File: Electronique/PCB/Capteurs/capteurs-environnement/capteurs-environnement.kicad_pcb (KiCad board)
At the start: 2 copper layers, 99.1 x 66 mm, 22 parts, among them U1 Pico

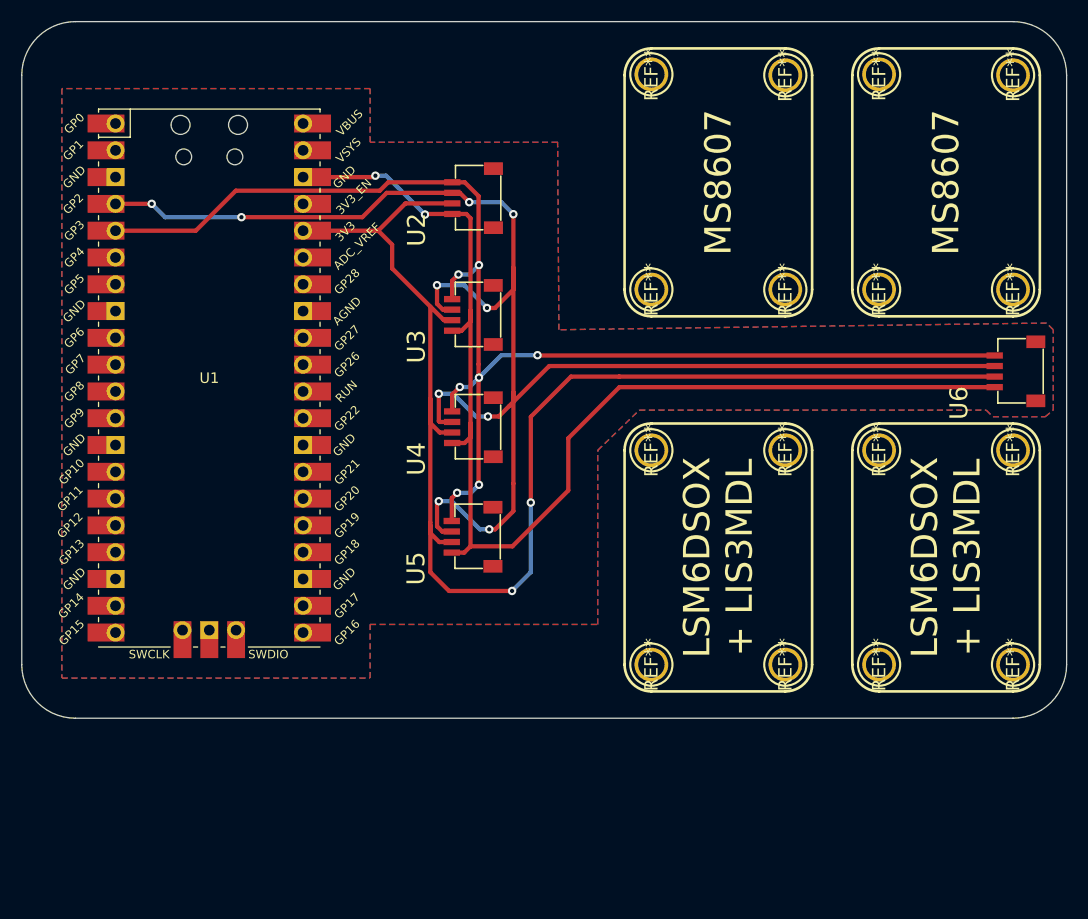
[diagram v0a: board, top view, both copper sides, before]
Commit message: pcb updates
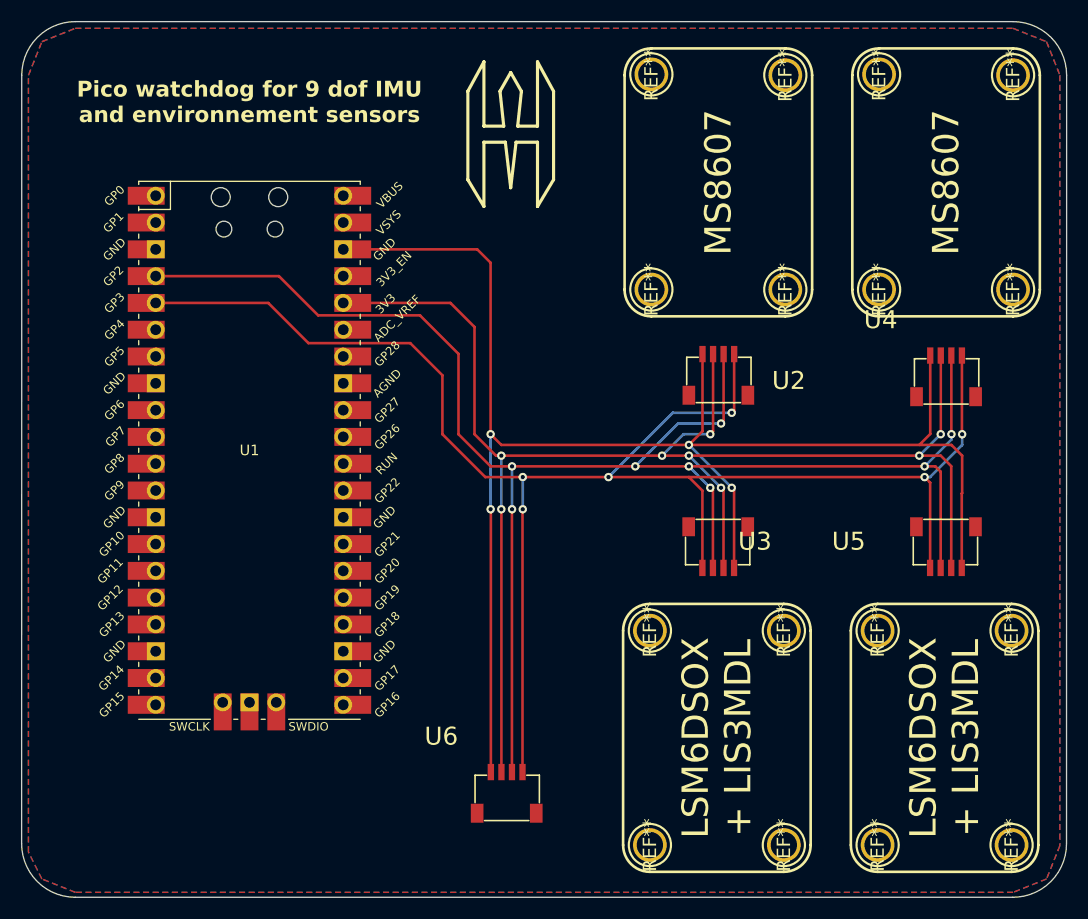
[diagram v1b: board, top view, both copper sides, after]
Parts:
- moved U6 63.4 mm to (110.7, 134.6), turned to 0 degrees
- moved U4 44.5 mm to (152.4, 95.1), turned to 0 degrees
- moved U5 44.3 mm to (152.4, 110.2), turned to 180 degrees
- moved U3 31.3 mm to (130.8, 110.2), turned to 180 degrees
- moved U2 28.5 mm to (130.8, 95.0), turned to 0 degrees
- moved REF** 17.1 mm to (137.0, 139.0)
- moved REF** 17.1 mm to (158.6, 139.0)
- moved REF** 17.1 mm to (124.3, 118.7)
- moved REF** 17.1 mm to (137.0, 118.7)
- moved REF** 17.1 mm to (145.9, 139.0)
- moved REF** 17.1 mm to (124.3, 139.0)
- moved REF** 17.1 mm to (145.9, 118.7)
- moved REF** 17.1 mm to (158.6, 118.7)
- moved U1 7.84 mm to (86.4, 101.6)
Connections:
- U2 pad MT1: GND -> unconnected-(U2-PadMT1)
- U2 pad MT2: GND -> unconnected-(U2-PadMT2)
- U3 pad MT1: GND -> unconnected-(U3-PadMT1)
- U3 pad MT2: GND -> unconnected-(U3-PadMT2)
- U4 pad MT1: GND -> unconnected-(U4-PadMT1)
- U4 pad MT2: GND -> unconnected-(U4-PadMT2)
- U5 pad MT1: GND -> unconnected-(U5-PadMT1)
- U5 pad MT2: GND -> unconnected-(U5-PadMT2)
- U6 pad MT1: GND -> unconnected-(U6-PadMT1)
- U6 pad MT2: GND -> unconnected-(U6-PadMT2)
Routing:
- net GND: track 116.2 -> 150.5 mm, vias 2 -> 4
- net /SCL: track 129.0 -> 162.1 mm, vias 7 -> 6
- net +3.3V: track 131.4 -> 145.1 mm, vias 2 -> 8
- net /SDA: track 155.9 -> 163.3 mm, vias 10 -> 8
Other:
- board size 99.1 x 66 mm -> 99.1 x 83 mm
- board text added: "Pico watchdog for 9 dof IMU and environnement sensors"
